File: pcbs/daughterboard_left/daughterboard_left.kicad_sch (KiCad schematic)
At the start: 4 parts, among them J1 Conn_01x10_Socket, J2 Conn_01x02, SW1 SW_SPST, U1 nice_nano

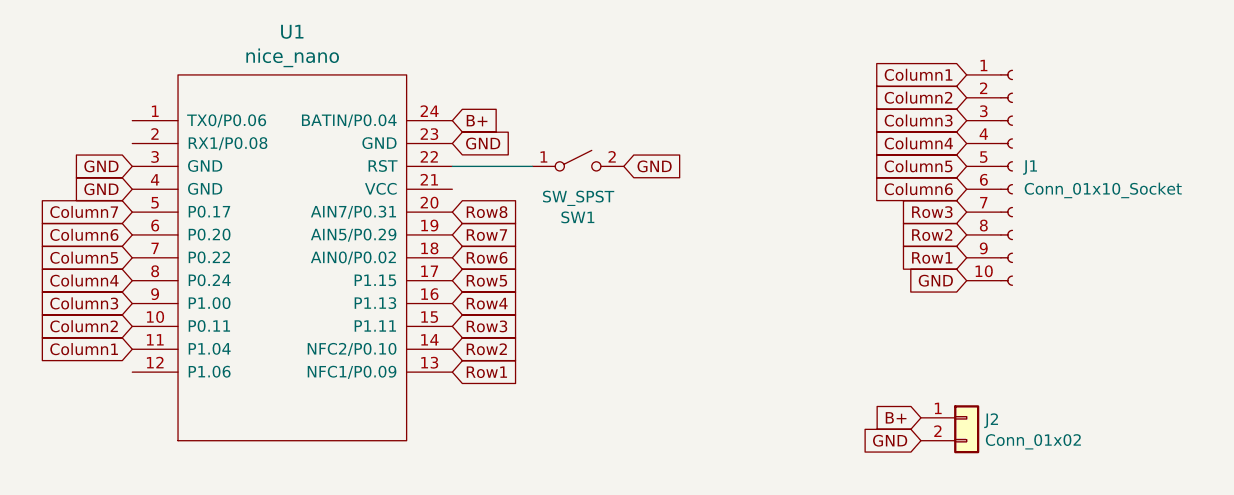
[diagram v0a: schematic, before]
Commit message: more changes
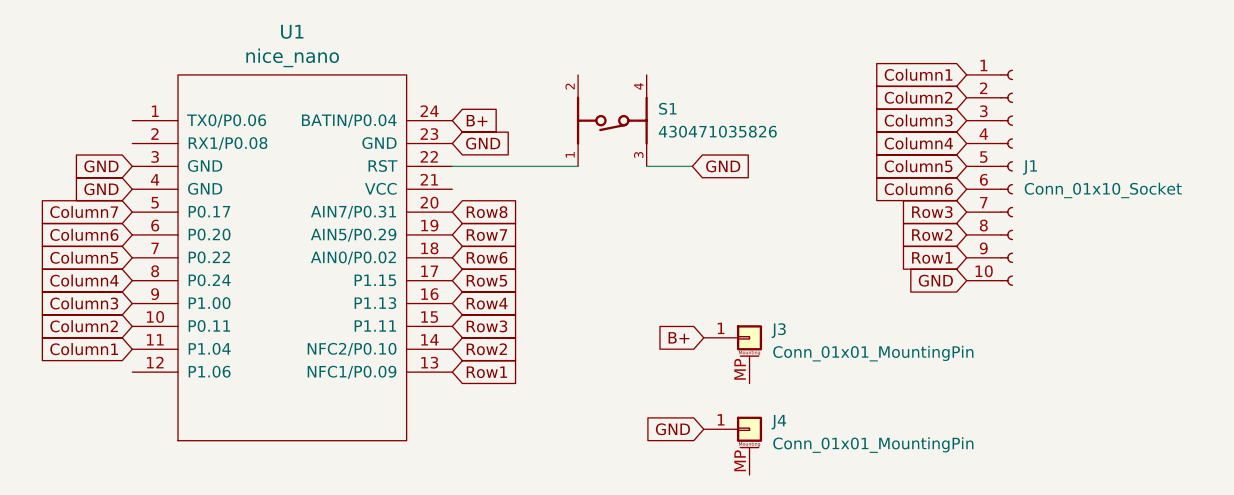
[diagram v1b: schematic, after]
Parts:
- removed J2: Conn_01x02, Connector_JST:JST_PH_S2B-PH-K_1x02_P2.00mm_Horizontal, symbol Connector_Generic:Conn_01x02
- removed SW1: SW_SPST, Button_Switch_THT:SW_Tactile_SPST_Angled_PTS645Vx83-2LFS, symbol Switch:SW_SPST
- added J3, J4: Conn_01x01_MountingPin, symbol Connector_Generic_MountingPin:Conn_01x01_MountingPin
- added S1: 430471035826, ResetSwitch:430471035826, symbol ResetSwitch:430471035826
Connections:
- net B+: now also J3.1 (Pin_1)
- net GND: now also J4.1 (Pin_1), S1.3
- net at U1.22 (RST): now also S1.1
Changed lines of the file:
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@@
 (kicad_sch (version 20230121) (generator eeschema)
   (paper "A4")
-  (wire (pts (xy 85.09 64.77) (xy 93.98 64.77))
+  (wire (pts (xy 85.09 64.77) (xy 99.06 64.77))
     (stroke (width 0) (type default))
   )
+  (wire (pts (xy 106.68 64.77) (xy 111.76 64.77))
+    (stroke (width 0) (type default))
+  )
   (global_label "Column1" (shape input) (at 49.53 85.09 180)
     (effects (font (size 1.27 1.27)) (justify right))
@@
     )
   )
-  (global_label "B+" (shape input) (at 137.16 92.71 180)
-    (effects (font (size 1.27 1.27)) (justify right))
-    (property "Intersheetrefs" "${INTERSHEET_REFS}" (at 137.16 92.71 0)
+  (global_label "B+" (shape input) (at 113.03 83.82 180)
+    (effects (font (size 1.27 1.27)) (justify right))
+    (property "Intersheetrefs" "${INTERSHEET_REFS}" (at 113.03 83.82 0)
       (effects (font (size 1.27 1.27)) hide)
     )
@@
     )
   )
-  (global_label "GND" (shape input) (at 137.16 95.25 180)
-    (effects (font (size 1.27 1.27)) (justify right))
-    (property "Intersheetrefs" "${INTERSHEET_REFS}" (at 137.16 95.25 0)
+  (global_label "GND" (shape input) (at 113.03 93.98 180)
+    (effects (font (size 1.27 1.27)) (justify right))
+    (property "Intersheetrefs" "${INTERSHEET_REFS}" (at 113.03 93.98 0)
       (effects (font (size 1.27 1.27)) hide)
     )
@@
     )
   )
-  (global_label "GND" (shape input) (at 104.14 64.77 0)
-    (effects (font (size 1.27 1.27)) (justify left))
-    (property "Intersheetrefs" "${INTERSHEET_REFS}" (at 104.14 64.77 0)
+  (global_label "GND" (shape input) (at 111.76 64.77 0)
+    (effects (font (size 1.27 1.27)) (justify left))
+    (property "Intersheetrefs" "${INTERSHEET_REFS}" (at 111.76 64.77 0)
       (effects (font (size 1.27 1.27)) hide)
     )
@@
     )
   )
-  (symbol (lib_id "Connector_Generic:Conn_01x02") (at 142.24 92.71 0) (unit 1)
-    (in_bom yes) (on_board yes) (dnp no)
-    (property "Reference" "J2" (at 144.272 92.9132 0)
-      (effects (font (size 1.27 1.27)) (justify left))
-    )
-    (property "Value" "Conn_01x02" (at 144.272 95.2246 0)
-      (effects (font (size 1.27 1.27)) (justify left))
-    )
-    (property "Footprint" "Connector_JST:JST_PH_S2B-PH-K_1x02_P2.00mm_Horizontal" (at 142.24 92.71 0)
-      (effects (font (size 1.27 1.27)) hide)
-    )
-    (property "Datasheet" "~" (at 142.24 92.71 0)
-      (effects (font (size 1.27 1.27)) hide)
+  (symbol (lib_id "Connector_Generic_MountingPin:Conn_01x01_MountingPin") (at 118.11 93.98 0) (unit 1)
+    (in_bom yes) (on_board yes) (dnp no) (fields_autoplaced)
+    (property "Reference" "J4" (at 120.65 93.0656 0)
+      (effects (font (size 1.27 1.27)) (justify left))
+    )
+    (property "Value" "Conn_01x01_MountingPin" (at 120.65 95.6056 0)
+      (effects (font (size 1.27 1.27)) (justify left))
+    )
+    (property "Footprint" "" (at 118.11 93.98 0)
+      (effects (font (size 1.27 1.27)) hide)
+    )
+    (property "Datasheet" "~" (at 118.11 93.98 0)
+      (effects (font (size 1.27 1.27)) hide)
+    )
+    (pin "1")
+    (pin "MP")
+    (instances
+      (project "daughterboard_left"
+        (path "/16085aa0-524e-4720-90a1-7a76115f3b87"
+          (reference "J4") (unit 1)
+        )
+      )
+    )
+  )
+  (symbol (lib_id "ResetSwitch:430471035826") (at 104.14 59.69 90) (unit 1)
+    (in_bom yes) (on_board yes) (dnp no) (fields_autoplaced)
+    (property "Reference" "S1" (at 107.95 58.42 90)
+      (effects (font (size 1.27 1.27)) (justify right))
+    )
+    (property "Value" "430471035826" (at 107.95 60.96 90)
+      (effects (font (size 1.27 1.27)) (justify right))
+    )
+    (property "Footprint" "ResetSwitch:430471035826" (at 104.14 59.69 0)
+      (effects (font (size 1.27 1.27)) (justify bottom) hide)
+    )
+    (property "Datasheet" "" (at 104.14 59.69 0)
+      (effects (font (size 1.27 1.27)) hide)
+    )
+    (property "MF" "Wurth Electronics Inc." (at 104.14 59.69 0)
+      (effects (font (size 1.27 1.27)) (justify bottom) hide)
+    )
+    (property "Description" "\nTactile Switch SPST-NO Top Actuated Surface Mount\n" (at 104.14 59.69 0)
+      (effects (font (size 1.27 1.27)) (justify bottom) hide)
+    )
+    (property "Package" "None" (at 104.14 59.69 0)
+      (effects (font (size 1.27 1.27)) (justify bottom) hide)
+    )
+    (property "Price" "None" (at 104.14 59.69 0)
+      (effects (font (size 1.27 1.27)) (justify bottom) hide)
+    )
+    (property "VALUE" "430471035826" (at 104.14 59.69 0)
+      (effects (font (size 1.27 1.27)) (justify bottom) hide)
+    )
+    (property "QTY" "2000" (at 104.14 59.69 0)
+      (effects (font (size 1.27 1.27)) (justify bottom) hide)
+    )
+    (property "SnapEDA_Link" "https://www.snapeda.com/parts/430471035826/Wurth+Electronics+Inc/view-part/?ref=snap" (at 104.14 59.69 0)
+      (effects (font (size 1.27 1.27)) (justify bottom) hide)
+    )
+    (property "DATASHEET-URL" "https://www.we-online.com/redexpert/spec/430471035826?ae" (at 104.14 59.69 0)
+      (effects (font (size 1.27 1.27)) (justify bottom) hide)
+    )
+    (property "MP" "430471035826" (at 104.14 59.69 0)
+      (effects (font (size 1.27 1.27)) (justify bottom) hide)
+    )
+    (property "PART-NUMBER" "430471035826" (at 104.14 59.69 0)
+      (effects (font (size 1.27 1.27)) (justify bottom) hide)
+    )
+    (property "OPERATION-FORCE" "260g" (at 104.14 59.69 0)
+      (effects (font (size 1.27 1.27)) (justify bottom) hide)
+    )
+    (property "HEIGHT" "3.5mm" (at 104.14 59.69 0)
+      (effects (font (size 1.27 1.27)) (justify bottom) hide)
+    )
+    (property "Availability" "In Stock" (at 104.14 59.69 0)
+      (effects (font (size 1.27 1.27)) (justify bottom) hide)
+    )
+    (property "Check_prices" "https://www.snapeda.com/parts/430471035826/Wurth+Electronics+Inc/view-part/?ref=eda" (at 104.14 59.69 0)
+      (effects (font (size 1.27 1.27)) (justify bottom) hide)
     )
     (pin "1")
     (pin "2")
-    (instances
-      (project "daughterboard_left"
-        (path "/16085aa0-524e-4720-90a1-7a76115f3b87"
-          (reference "J2") (unit 1)
-        )
-      )
-    )
-  )
-  (symbol (lib_id "Switch:SW_SPST") (at 99.06 64.77 0) (unit 1)
-    (in_bom yes) (on_board yes) (dnp no)
-    (property "Reference" "SW1" (at 99.06 70.485 0)
-      (effects (font (size 1.27 1.27)))
-    )
-    (property "Value" "SW_SPST" (at 99.06 68.1736 0)
-      (effects (font (size 1.27 1.27)))
-    )
-    (property "Footprint" "Button_Switch_THT:SW_Tactile_SPST_Angled_PTS645Vx83-2LFS" (at 99.06 64.77 0)
-      (effects (font (size 1.27 1.27)) hide)
-    )
-    (property "Datasheet" "~" (at 99.06 64.77 0)
-      (effects (font (size 1.27 1.27)) hide)
-    )
-    (pin "1")
-    (pin "2")
-    (instances
-      (project "daughterboard_left"
-        (path "/16085aa0-524e-4720-90a1-7a76115f3b87"
-          (reference "SW1") (unit 1)
+    (pin "3")
+    (pin "4")
+    (instances
+      (project "daughterboard_left"
+        (path "/16085aa0-524e-4720-90a1-7a76115f3b87"
+          (reference "S1") (unit 1)
         )
       )
@@
         )
       )
+    )
+  )
+  (symbol (lib_id "Connector_Generic_MountingPin:Conn_01x01_MountingPin") (at 118.11 83.82 0) (unit 1)
+    (in_bom yes) (on_board yes) (dnp no) (fields_autoplaced)
+    (property "Reference" "J3" (at 120.65 82.9056 0)
+      (effects (font (size 1.27 1.27)) (justify left))
+    )
+    (property "Value" "Conn_01x01_MountingPin" (at 120.65 85.4456 0)
+      (effects (font (size 1.27 1.27)) (justify left))
+    )
+    (property "Footprint" "" (at 118.11 83.82 0)
+      (effects (font (size 1.27 1.27)) hide)
+    )
+    (property "Datasheet" "~" (at 118.11 83.82 0)
+      (effects (font (size 1.27 1.27)) hide)
+    )
+    (pin "1")
+    (pin "MP")
+    (instances
+      (project "daughterboard_left"
+        (path "/16085aa0-524e-4720-90a1-7a76115f3b87"
+          (reference "J3") (unit 1)
+        )
+      )
